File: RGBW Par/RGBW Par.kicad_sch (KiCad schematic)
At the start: 2 parts, among them J1 530470410, U1 ATtiny84-20M

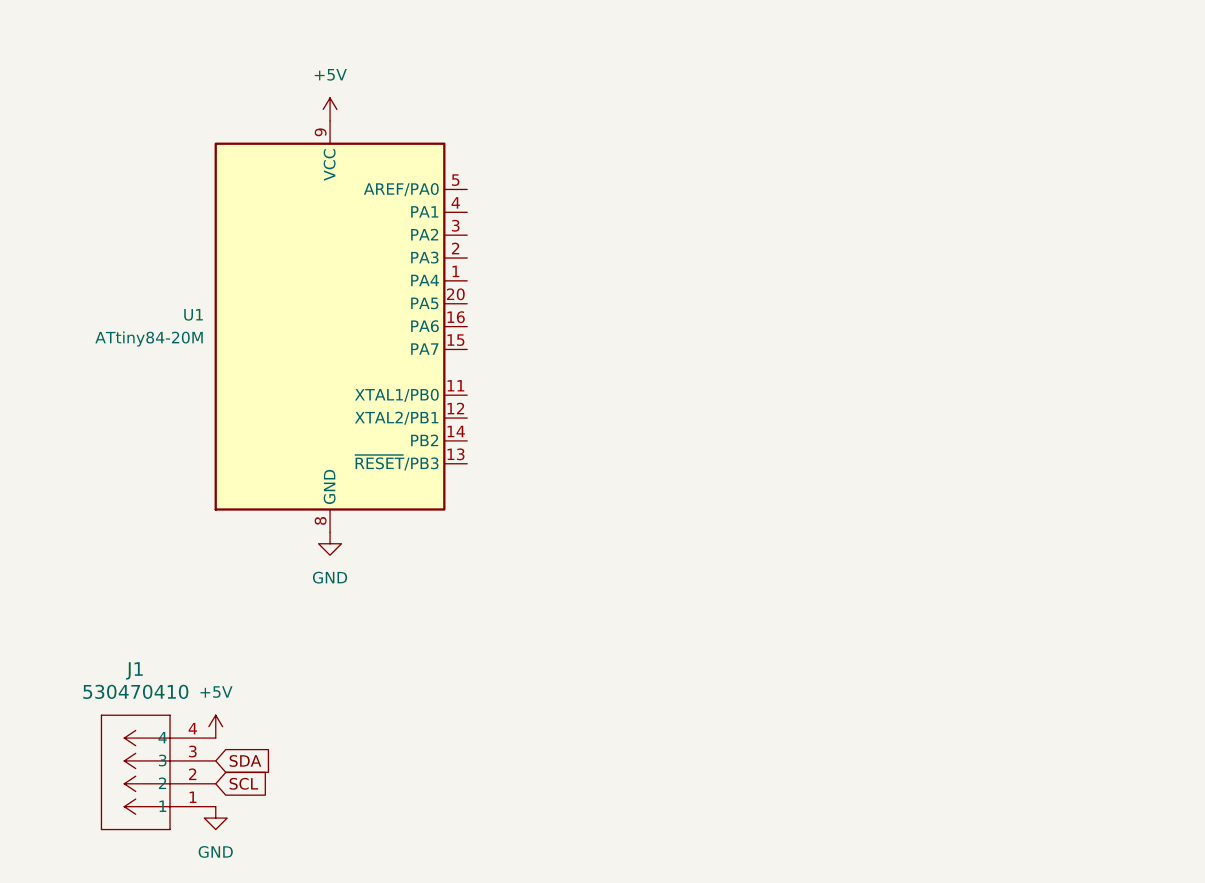
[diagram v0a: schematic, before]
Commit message: RGB Par V1
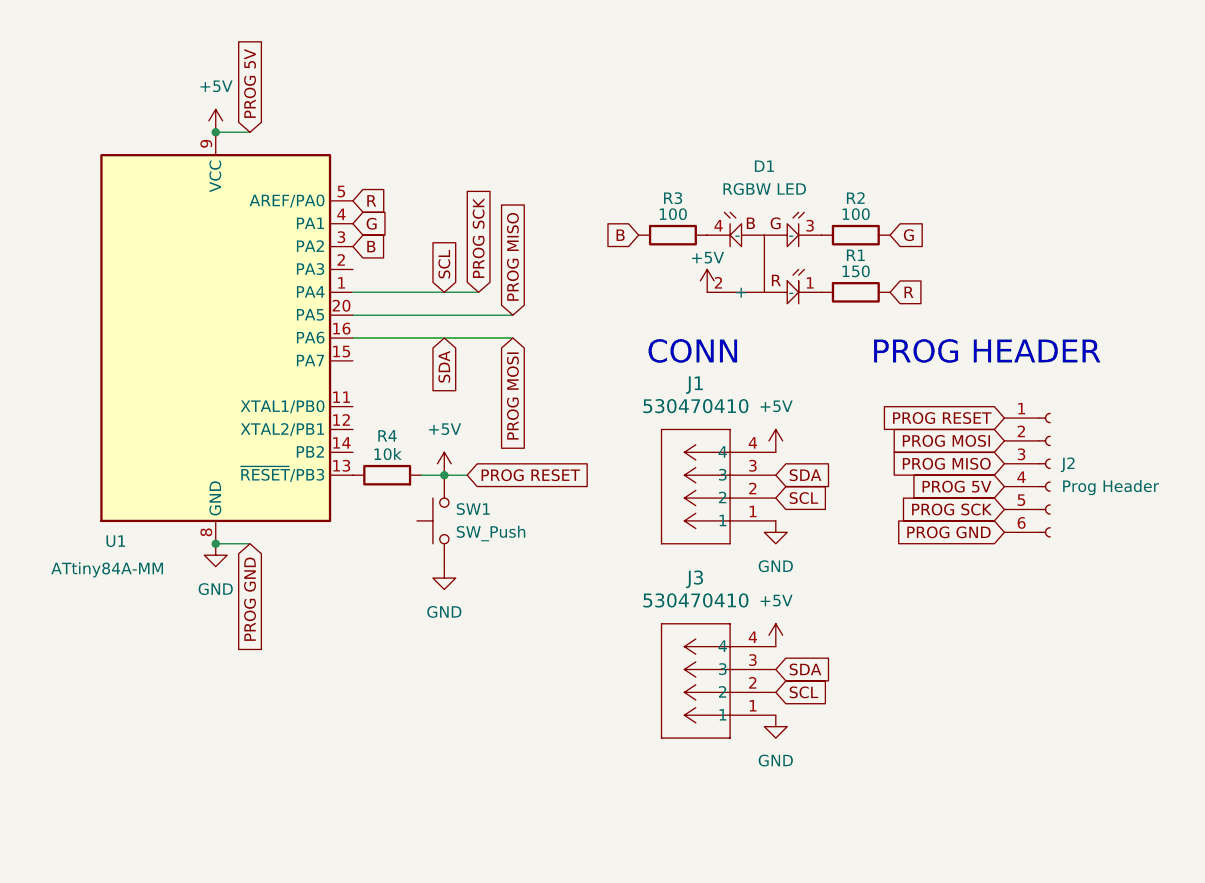
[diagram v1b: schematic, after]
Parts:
- removed U1: ATtiny84-20M, Package_DFN_QFN:QFN-20-1EP_4x4mm_P0.5mm_EP2.6x2.6mm, symbol MCU_Microchip_ATtiny:ATtiny84-20M
- added D1: RGBW LED, XL-3528RGBW-HM:XL-3528RGBW-HM, symbol XL-3528RGBW-HM:XL-3528RGBW-HM
- added J2: Prog Header, Connector_PinHeader_2.54mm:PinHeader_1x06_P2.54mm_Vertical, symbol Connector:Conn_01x06_Socket
- added J3: 530470410, Connector_Molex:Molex_PicoBlade_53047-0410_1x04_P1.25mm_Vertical, symbol CONN04_530470410_MOL:530470410
- added R1: 150, Resistor_SMD:R_0201_0603Metric, symbol Device:R
- added R2, R3: 100, Resistor_SMD:R_0201_0603Metric, symbol Device:R
- added R4: 10k, Resistor_SMD:R_0201_0603Metric, symbol Device:R
- added SW1: SW_Push, Connector_PinHeader_2.54mm:PinHeader_1x02_P2.54mm_Vertical, symbol Switch:SW_Push
- added U1: ATtiny84A-MM, Package_DFN_QFN:QFN-20-1EP_3x3mm_P0.45mm_EP1.6x1.6mm, symbol MCU_Microchip_ATtiny:ATtiny84A-MM
- J1: footprint CONN04_530470410_MOL -> Connector_Molex:Molex_PicoBlade_53047-0410_1x04_P1.25mm_Vertical
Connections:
- net +5V: now also D1.2 (+), J2.1 (Pin_1), J2.4 (Pin_4), J3.4, R4.2, SW1.2, U1.9 (VCC)
- net GND: now also J2.6 (Pin_6), J3.1, SW1.1, U1.21 (GND), U1.8 (GND)
- net SCL renamed PROG SCK
- net PROG SCK: now also J2.5 (Pin_5), J3.2, U1.1 (PA4)
- net SDA renamed PROG MOSI
- net PROG MOSI: now also J2.2 (Pin_2), J3.3, U1.16 (PA6)
- new net: D1.1 (-), R1.2
- new net: D1.3 (-), R2.2
- new net: D1.4 (-), R3.1
- new net: R4.1, U1.13 (~{RESET}/PB3)
- new net B: R3.2, U1.3 (PA2)
- new net G: R2.1, U1.4 (PA1)
- new net PROG MISO: J2.3 (Pin_3), U1.20 (PA5)
- new net R: R1.1, U1.5 (AREF/PA0)
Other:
- note added: "CONN"
- note added: "PROG HEADER"
- moved on the sheet: J1

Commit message: rgb par v2
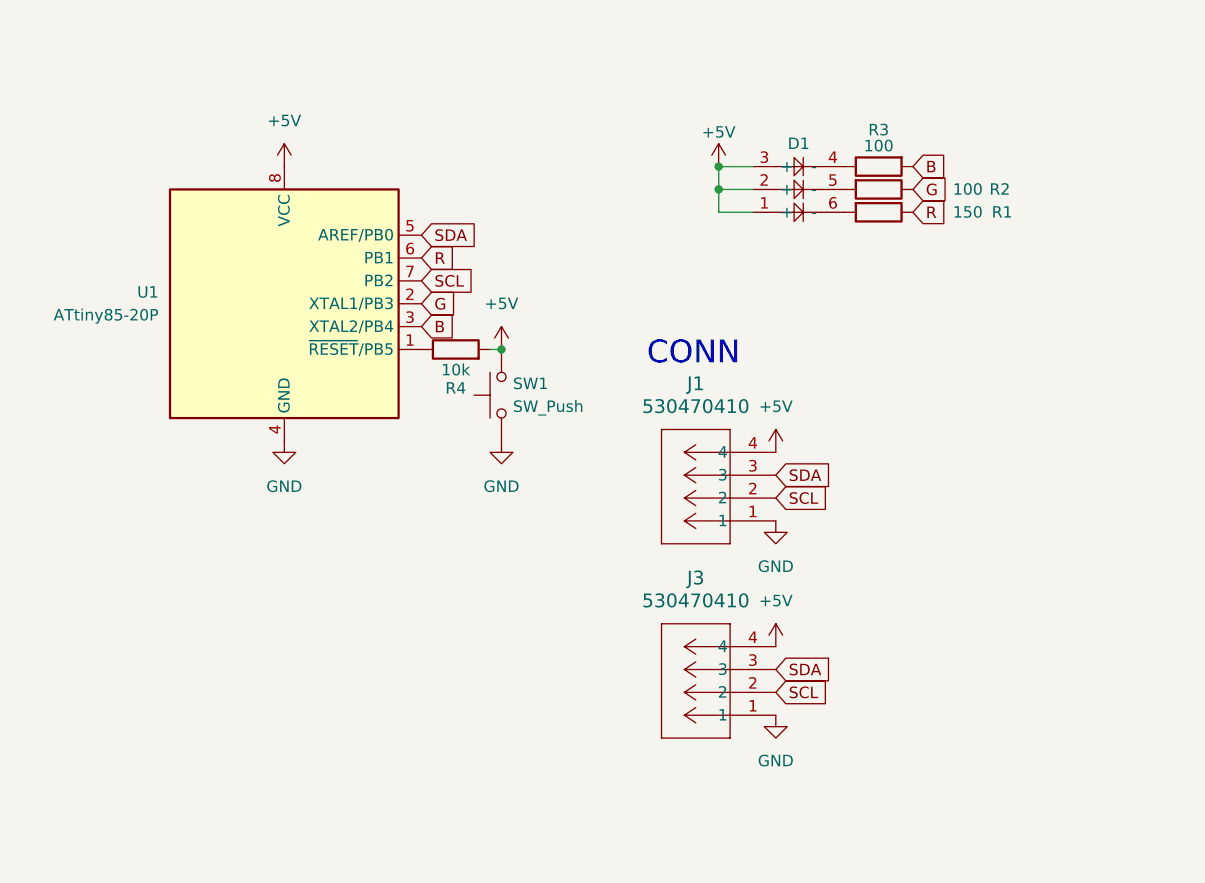
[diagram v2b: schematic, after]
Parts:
- removed D1: RGBW LED, XL-3528RGBW-HM:XL-3528RGBW-HM, symbol XL-3528RGBW-HM:XL-3528RGBW-HM
- removed J2: Prog Header, Connector_PinHeader_2.54mm:PinHeader_1x06_P2.54mm_Vertical, symbol Connector:Conn_01x06_Socket
- removed U1: ATtiny84A-MM, Package_DFN_QFN:QFN-20-1EP_3x3mm_P0.45mm_EP1.6x1.6mm, symbol MCU_Microchip_ATtiny:ATtiny84A-MM
- added D1: ~, RGB_LED:rgb_led, symbol rgb_led:rgb_led
- added U1: ATtiny85-20P, Package_DIP:DIP-8_W7.62mm, symbol MCU_Microchip_ATtiny:ATtiny85-20P
- R1, R2, R3, R4: footprint Resistor_SMD:R_0201_0603Metric -> Resistor_THT:R_Axial_DIN0207_L6.3mm_D2.5mm_P7.62mm_Horizontal
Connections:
- net +5V: now also D1.1 (+), D1.2 (+), D1.3 (+), U1.8 (VCC)
- net B: now also U1.3 (XTAL2/PB4)
- net G: now also U1.2 (XTAL1/PB3)
- net GND: now also U1.4 (GND)
- net R: now also U1.6 (PB1)
- net at R1.2: now also D1.6 (-)
- net at R2.2: now also D1.5 (-)
- net at R3.1: now also D1.4 (-)
- net at R4.1: now also U1.1 (~{RESET}/PB5)
- net PROG MOSI renamed SDA
- net SDA: now also U1.5 (AREF/PB0)
- net PROG SCK renamed SCL
- net SCL: now also U1.7 (PB2)
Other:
- note removed: "PROG HEADER"
- moved on the sheet: R1, R2, R3, R4, SW1
